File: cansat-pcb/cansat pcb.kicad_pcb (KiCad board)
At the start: 2 copper layers, 74 x 214 mm, 19 parts, among them J1 Conn_01x03_Pin, J2 Conn_01x03_Pin, J3 Conn_01x03_Pin, Q1 2N3904, Q2 AO3400A, SW1 SW_DPDT_x2, U3 MPU6050

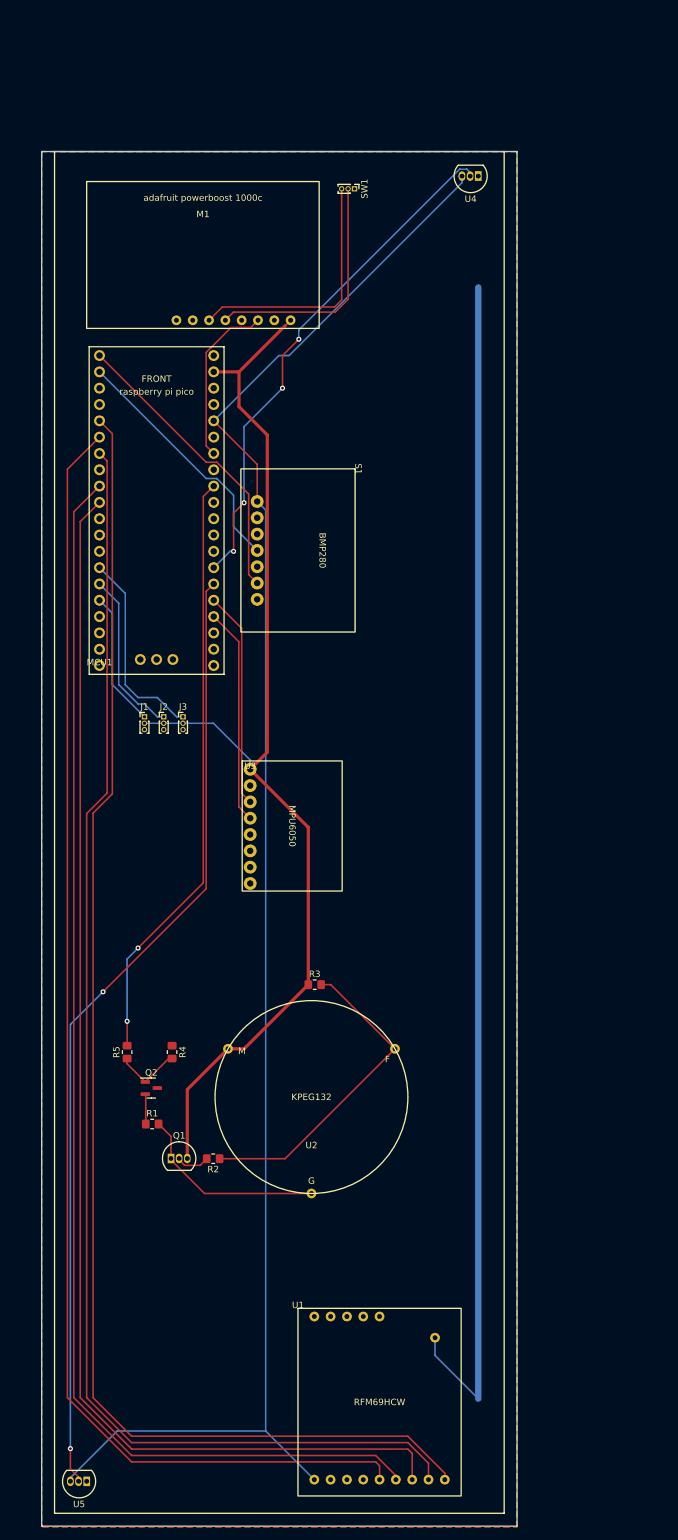
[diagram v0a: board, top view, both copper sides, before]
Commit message: made some changes to pcb (fuck you Berenger)
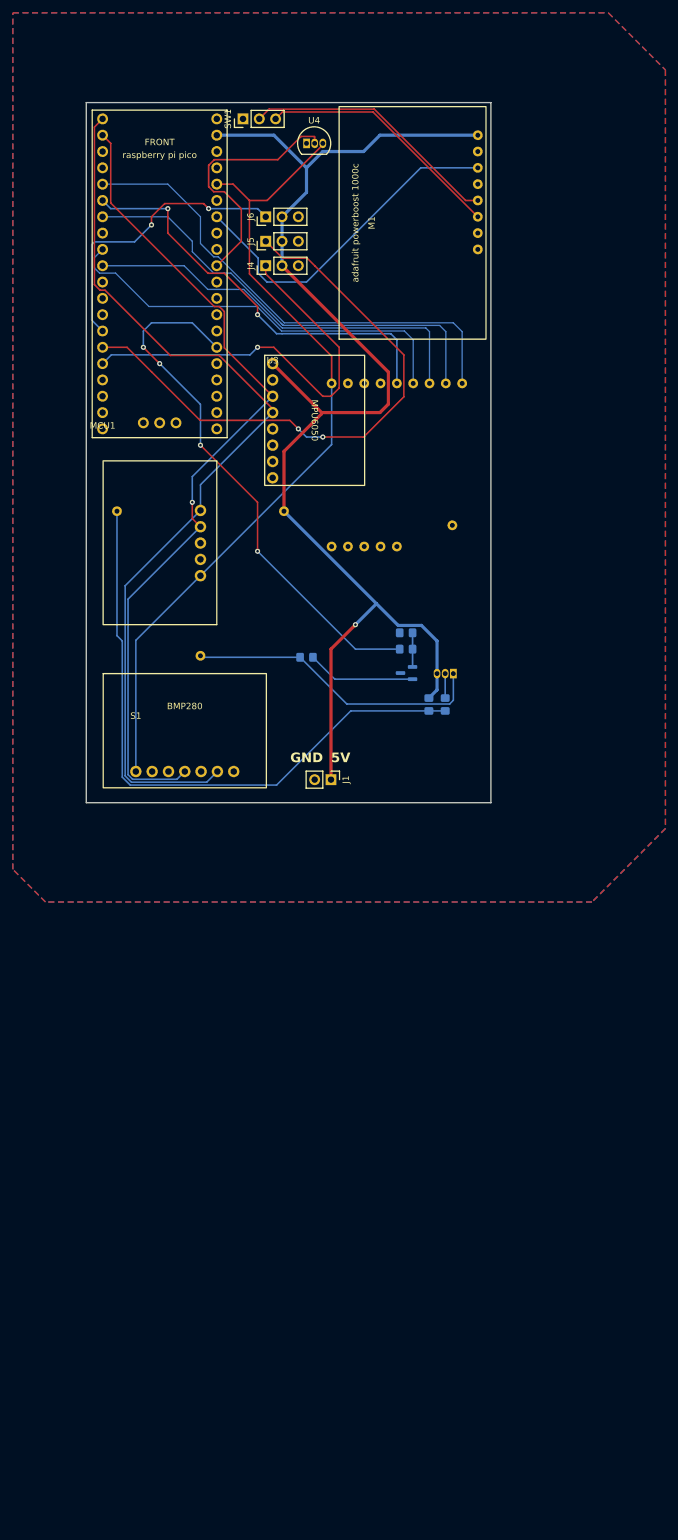
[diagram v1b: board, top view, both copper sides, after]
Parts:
- removed J2, J3: Conn_01x03_Pin, Connector_PinHeader_1.00mm:PinHeader_1x03_P1.00mm_Vertical
- added J4: Conn_01x03_Pin, Connector_PinHeader_2.54mm:PinHeader_1x03_P2.54mm_Vertical, F.Cu at (153.9, 65.4)
- added J5: Conn_01x03_Pin, Connector_PinHeader_2.54mm:PinHeader_1x03_P2.54mm_Vertical, F.Cu at (153.9, 61.6)
- added J6: Conn_01x03_Pin, Connector_PinHeader_2.54mm:PinHeader_1x03_P2.54mm_Vertical, F.Cu at (153.9, 57.8)
- J1: value Conn_01x03_Pin -> Conn_01x02_Pin; footprint Connector_PinHeader_1.00mm:PinHeader_1x03_P1.00mm_Vertical -> Connector_PinHeader_2.54mm:PinHeader_1x02_P2.54mm_Vertical
- Q1: value 2N3904 -> AO3400A; footprint Package_TO_SOT_THT:TO-92_Inline -> Package_TO_SOT_SMD:SOT-23; moved to B.Cu
- Q2: value AO3400A -> 2N3904; footprint Package_TO_SOT_SMD:SOT-23 -> Package_TO_SOT_THT:TO-92_Inline; moved to B.Cu
- R1: value 1K -> 100K; moved to B.Cu
- R2: value 22K -> 1K; moved to B.Cu
- R3: value 100K -> 1K; moved to B.Cu
- R4, U1, U2: moved to B.Cu
- R5: value 1K -> 22K; moved to B.Cu
- SW1: footprint Connector_PinHeader_1.00mm:PinHeader_1x03_P1.00mm_Vertical -> Connector_PinHeader_2.54mm:PinHeader_1x03_P2.54mm_Vertical
- U5: value ~ -> SGP30; footprint Package_TO_SOT_THT:TO-92L_Inline -> CanSat:SGP30
- moved U5 142.1 mm to (143.8, 113.7), turned to 90 degrees
- moved U1 117.4 mm to (161.7, 110.4)
- moved R1 86.1 mm to (175.8, 122.5)
- moved U2 85.5 mm to (143.8, 111.1), turned to 180 degrees
- moved R2 84.8 mm to (175.8, 125.1)
- moved Q1 84.0 mm to (175.9, 128.8), turned to 180 degrees
- moved Q2 79.8 mm to (183.2, 128.9), turned to 180 degrees
- moved R5 73.4 mm to (181.9, 133.7)
- moved R4 67.3 mm to (179.3, 133.7)
- moved U3 63.2 mm to (155.0, 80.6)
- moved R3 51.0 mm to (160.3, 126.4), turned to 180 degrees
- moved S1 50.5 mm to (128.6, 128.9), turned to 0 degrees
- moved M1 46.3 mm to (165.4, 76.8), turned to 90 degrees
- moved MCU1 36.8 mm to (128.5, 90.8)
- moved J1 30.6 mm to (164.1, 145.4), turned to -90 degrees
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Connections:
- J1 pad 1: SERVO_1 -> +5V
- J1 pad 2: +5V -> GND
- MCU1 pad 24: I2C1 SDA -> unconnected-(MCU1-GP18-Pad24)
- MCU1 pad 25: I2C1 SCL -> unconnected-(MCU1-GP19-Pad25)
- MCU1 pad 26: TMP36_2 -> /buzzer
- MCU1 pad 27: TMP36_1 -> unconnected-(MCU1-GP21-Pad27)
- MCU1 pad 31: unconnected-(MCU1-GP26-Pad31) -> TMP1
- MCU1 pad 32: BUZZER -> unconnected-(MCU1-GP27-Pad32)
- MCU1 pad 5: SERVO_1 -> /SERVO/SERVO 1
- MCU1 pad 6: SERVO_2 -> /SERVO/SERVO 2
- MCU1 pad 7: SERVO_3 -> /SERVO/SERVO 3
- Q1 pad 1: Net-(Q1-E) -> Net-(Q1-G)
- Q1 pad 2: Net-(Q1-B) -> Net-(Q1-S)
- Q1 pad 3: +5V -> GND
- Q2 pad 1: Net-(Q2-G) -> Net-(Q2-E)
- Q2 pad 2: Net-(Q2-S) -> Net-(Q2-B)
- Q2 pad 3: GND -> +5V
- R1 pad 1: Net-(Q2-S) -> GND
- R1 pad 2: Net-(Q1-E) -> Net-(Q1-G)
- R2 pad 1: Net-(U2-F) -> Net-(Q1-G)
- R2 pad 2: Net-(Q1-B) -> /buzzer
- R3 pad 1: +5V -> Net-(Q1-S)
- R3 pad 2: Net-(U2-F) -> Net-(Q2-E)
- R4 pad 1: GND -> +5V
- R4 pad 2: Net-(Q2-G) -> Net-(U2-F)
- R5 pad 1: Net-(Q2-G) -> Net-(U2-F)
- R5 pad 2: BUZZER -> Net-(Q2-B)
- U2 pad 3: Net-(Q1-E) -> Net-(Q2-E)
- U3 pad 3: I2C1 SCL -> I2C0 SCL
- U3 pad 4: I2C1 SDA -> I2C0 SDA
- U4 pad 2: TMP36_1 -> TMP1
- U5 pad 1: GND -> +3V3
- U5 pad 2: TMP36_2 -> unconnected-(U5-1V8-Pad2)
- U5 pad 3: +3V3 -> GND
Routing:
- net unconnected-(U1-FM-Pad15): track 185.3 -> 0.00 mm
- net TMP36_2: track 149.5 -> 0.00 mm, vias 2 -> 0
- net SCK: track 206.8 -> 64.6 mm, vias 0 -> 2
- net RST: track 214.8 -> 76.0 mm
- net CS: track 208.8 -> 70.3 mm
- net MOSI: track 200.0 -> 63.2 mm
- net MISO: track 199.4 -> 64.5 mm
- net +3V3: track 260.9 -> 128.2 mm
- net I2C0 SDA: track 46.6 -> 144.2 mm
- net BUZZER: track 92.7 -> 0.00 mm, vias 2 -> 0
- net I2C0 SCL: track 38.9 -> 131.0 mm, vias 0 -> 1
- net /SERVO/SERVO 2: track 0.00 -> 90.6 mm, vias 0 -> 2
- net /buzzer: track 0.00 -> 83.6 mm, vias 0 -> 4
- net TMP36_1: track 80.6 -> 0.00 mm, vias 4 -> 0
- net /SERVO/SERVO 1: track 0.00 -> 65.3 mm, vias 0 -> 1
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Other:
- board size 74 x 214 mm -> 63 x 109 mm
- board text added: "5V"
- board text added: "GND"
